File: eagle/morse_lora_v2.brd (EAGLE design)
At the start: 55 x 82.9 mm, 20 parts

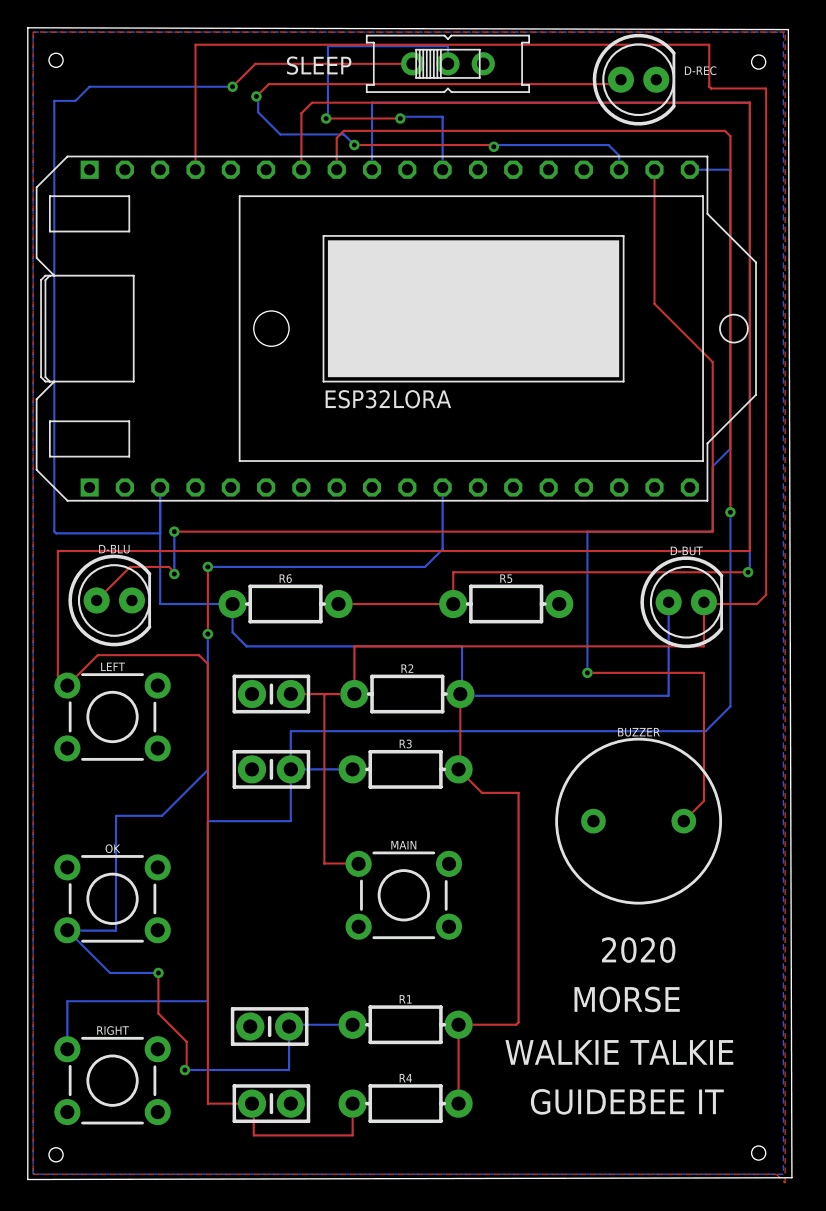
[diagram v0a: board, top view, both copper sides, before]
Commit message: update pcb v2
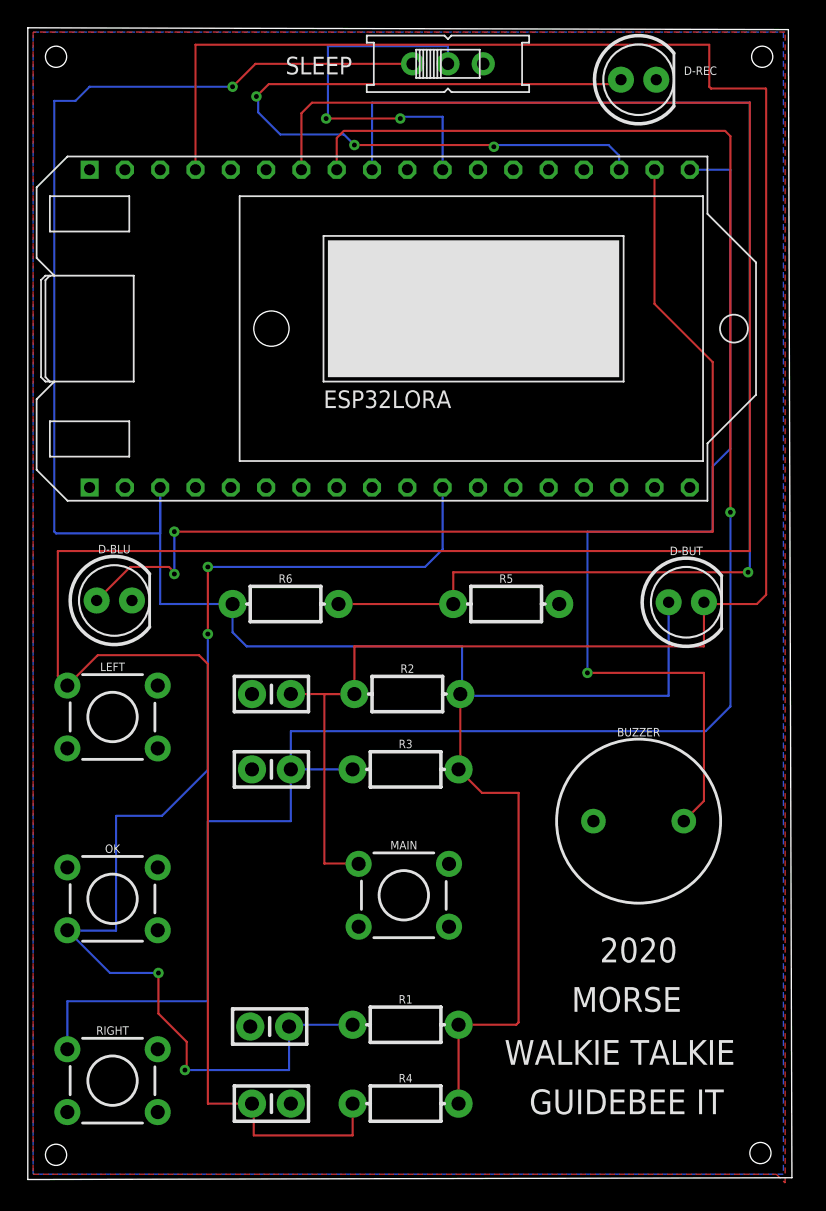
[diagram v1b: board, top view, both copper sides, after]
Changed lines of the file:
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@@
 <wire x1="54.082" y1="100.889" x2="-0.635" y2="101.016" width="0" layer="20"/>
 <wire x1="-0.635" y1="101.016" x2="-0.635" y2="18.161" width="0" layer="20"/>
-<hole x="1.397" y="98.679" drill="1.016"/>
-<hole x="51.943" y="98.552" drill="1.016"/>
-<hole x="51.943" y="20.066" drill="1.016"/>
-<hole x="1.397" y="19.939" drill="1.016"/>
+<hole x="1.397" y="98.933" drill="1.524"/>
+<hole x="52.197" y="98.933" drill="1.524"/>
+<hole x="52.07" y="20.066" drill="1.524"/>
+<hole x="1.397" y="19.939" drill="1.524"/>
 <hole x="16.891" y="79.375" drill="2.54"/>
 <text x="35.433" y="22.86" size="1.778" layer="25">GUIDEBEE IT</text>
